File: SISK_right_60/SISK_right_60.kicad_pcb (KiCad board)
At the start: 2 copper layers, 194.5 x 121.8 mm, 76 parts, among them J1 OLED_128x32, J2 Battery Conn, J3 alternative on/off SW (wired), SW1 "6", SW10 "Z", SW11 "U", SW12 "I", SW13 "O", SW14 "P", SW15 "Ü", SW16 "*", SW19 "H", SW2 "7", SW20 "J", SW21 "K", SW22 "L", SW23 "Ö", SW24 "Ä", SW25 "'", SW27 "N", SW28 "M", SW29 ";", SW3 "8", SW30 ":", SW31 "-", SW32 "shift_R", SW35 "SPACE_R", SW36 "Alt", SW37 FN, SW38 "Ctrl", SW39 FN2, SW4 "9", SW5 "0", SW6 "ß", SW7 "`", SW8 "Backspace", SW9 "Enter", U1 Nice_Nano_V2

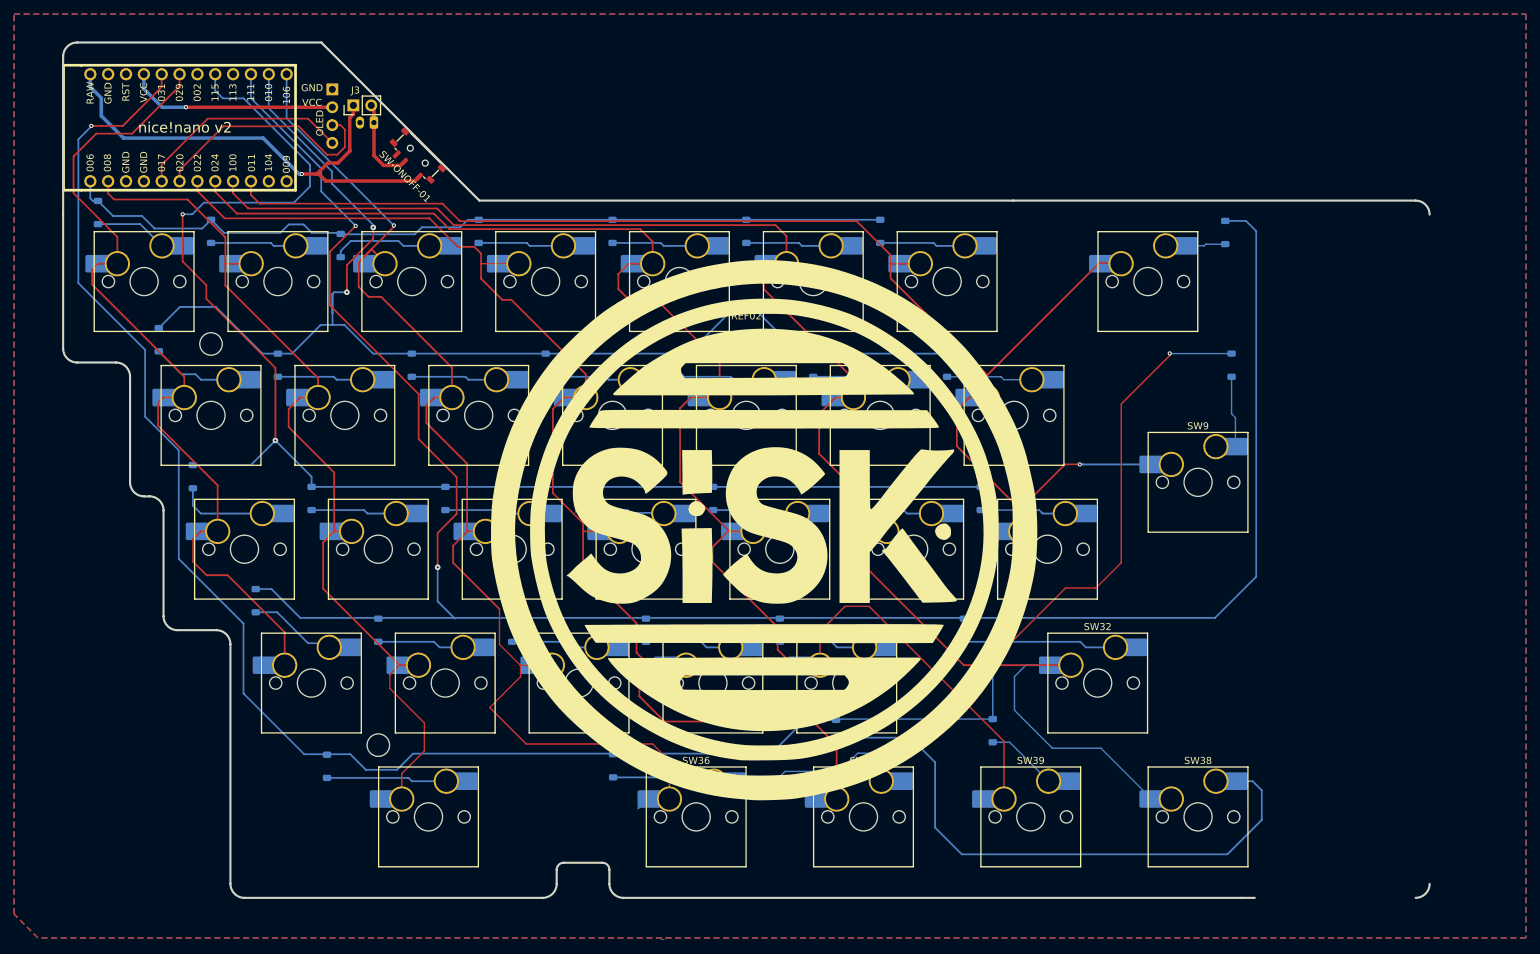
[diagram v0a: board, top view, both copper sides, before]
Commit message: fixed most of issues, updated 60% version
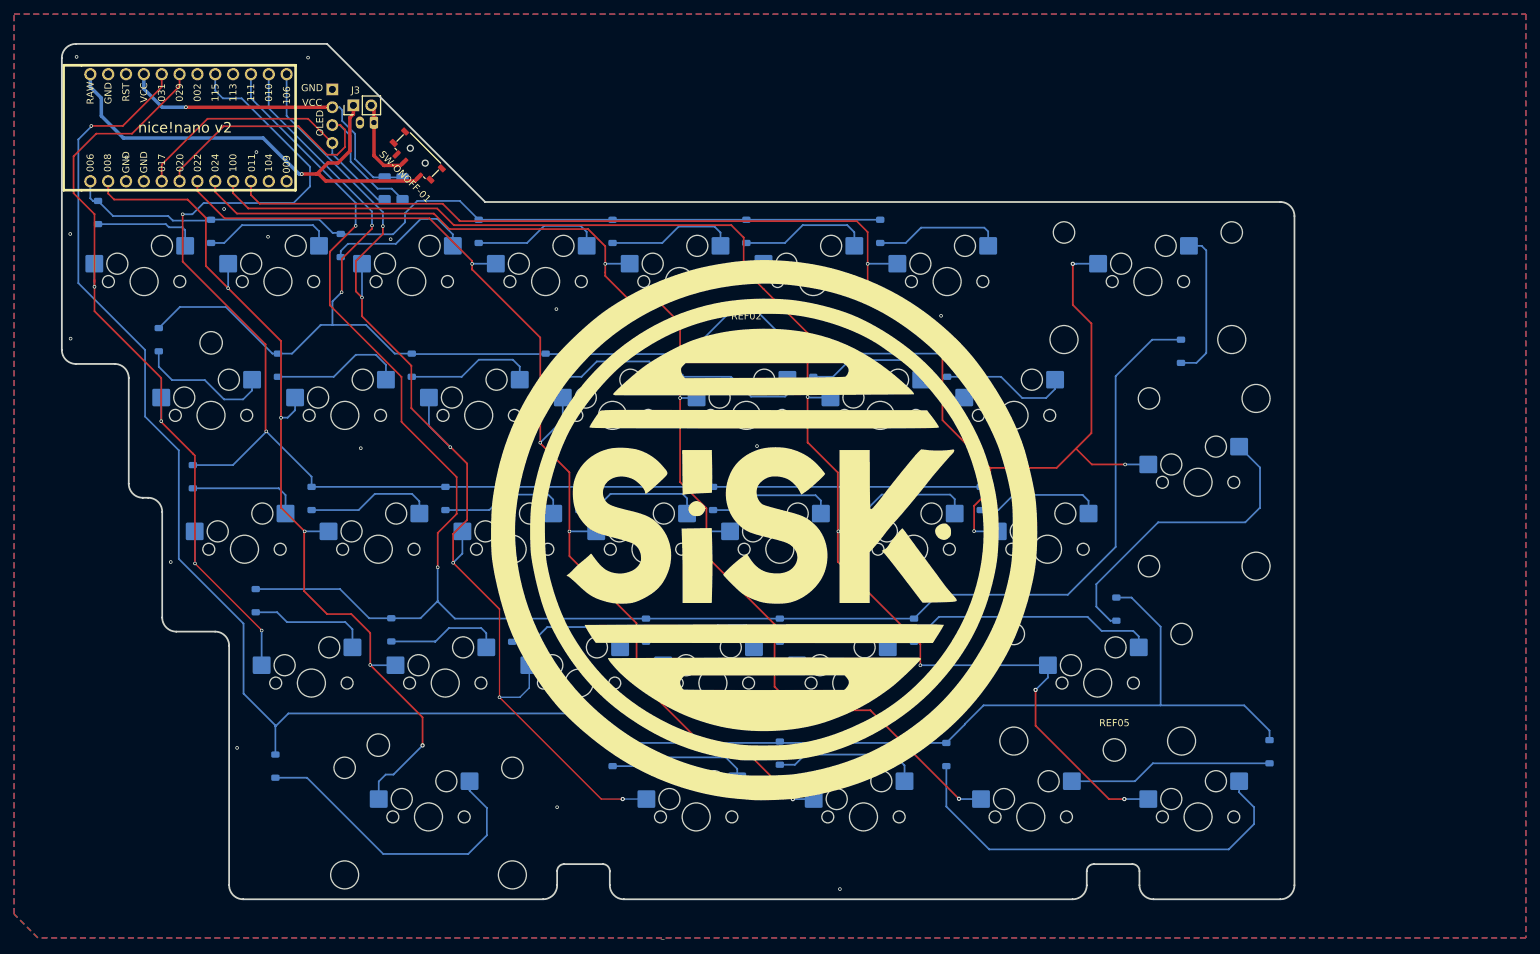
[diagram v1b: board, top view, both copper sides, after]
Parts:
- removed SW39: FN2, ScottoKeebs_Hotswap:Hotswap_MX_Plated_1.25u
- added R1: 5K, Resistor_SMD:R_1206_3216Metric_Pad1.30x1.75mm_HandSolder, B.Cu at (86.7, 51.8)
- added R2: 5K, Resistor_SMD:R_1206_3216Metric_Pad1.30x1.75mm_HandSolder, B.Cu at (89.2, 51.8)
- added REF05: MountingHole_3.2mm_M3_ISO7380, MountingHole:MountingHole_3.2mm_M3_ISO7380, F.Cu at (190.6, 131.7)
- added SW17: SW_push, MX_Hotswap:MX-Hotswap-1.25U, B.Cu at (178.7, 141.2)
- J2: value Battery Conn -> Conn
- J3: value alternative on/off SW (wired) -> SWITCH
- SW-ONOFF-01: value onboard ON/OFF SW -> ~
- SW1: value "6" -> SW_push; footprint ScottoKeebs_Hotswap:Hotswap_MX_Plated_1.00u -> MX_Hotswap:MX-Hotswap-1U; moved to B.Cu
- SW10: value "Z" -> SW_push; footprint ScottoKeebs_Hotswap:Hotswap_MX_Plated_1.00u -> MX_Hotswap:MX-Hotswap-1U; moved to B.Cu
- SW11: value "U" -> SW_push; footprint ScottoKeebs_Hotswap:Hotswap_MX_Plated_1.00u -> MX_Hotswap:MX-Hotswap-1U; moved to B.Cu
- SW12: value "I" -> SW_push; footprint ScottoKeebs_Hotswap:Hotswap_MX_Plated_1.00u -> MX_Hotswap:MX-Hotswap-1U; moved to B.Cu
- SW13: value "O" -> SW_push; footprint ScottoKeebs_Hotswap:Hotswap_MX_Plated_1.00u -> MX_Hotswap:MX-Hotswap-1U; moved to B.Cu
- SW14: value "P" -> SW_push; footprint ScottoKeebs_Hotswap:Hotswap_MX_Plated_1.00u -> MX_Hotswap:MX-Hotswap-1U; moved to B.Cu
- SW15: value "Ü" -> SW_push; footprint ScottoKeebs_Hotswap:Hotswap_MX_Plated_1.00u -> MX_Hotswap:MX-Hotswap-1U; moved to B.Cu
- SW16: value "*" -> SW_push; footprint ScottoKeebs_Hotswap:Hotswap_MX_Plated_1.00u -> MX_Hotswap:MX-Hotswap-1U; moved to B.Cu
- SW19: value "H" -> SW_push; footprint ScottoKeebs_Hotswap:Hotswap_MX_Plated_1.00u -> MX_Hotswap:MX-Hotswap-1U; moved to B.Cu
- SW2: value "7" -> SW_push; footprint ScottoKeebs_Hotswap:Hotswap_MX_Plated_1.00u -> MX_Hotswap:MX-Hotswap-1U; moved to B.Cu
- SW20: value "J" -> SW_push; footprint ScottoKeebs_Hotswap:Hotswap_MX_Plated_1.00u -> MX_Hotswap:MX-Hotswap-1U; moved to B.Cu
- SW21: value "K" -> SW_push; footprint ScottoKeebs_Hotswap:Hotswap_MX_Plated_1.00u -> MX_Hotswap:MX-Hotswap-1U; moved to B.Cu
- SW22: value "L" -> SW_push; footprint ScottoKeebs_Hotswap:Hotswap_MX_Plated_1.00u -> MX_Hotswap:MX-Hotswap-1U; moved to B.Cu
- SW23: value "Ö" -> SW_push; footprint ScottoKeebs_Hotswap:Hotswap_MX_Plated_1.00u -> MX_Hotswap:MX-Hotswap-1U; moved to B.Cu
- SW24: value "Ä" -> SW_push; footprint ScottoKeebs_Hotswap:Hotswap_MX_Plated_1.00u -> MX_Hotswap:MX-Hotswap-1U; moved to B.Cu
- SW25: value "'" -> SW_push; footprint ScottoKeebs_Hotswap:Hotswap_MX_Plated_1.00u -> MX_Hotswap:MX-Hotswap-1U; moved to B.Cu
- SW27: value "N" -> SW_push; footprint ScottoKeebs_Hotswap:Hotswap_MX_Plated_1.00u -> MX_Hotswap:MX-Hotswap-1U; moved to B.Cu
- SW28: value "M" -> SW_push; footprint ScottoKeebs_Hotswap:Hotswap_MX_Plated_1.00u -> MX_Hotswap:MX-Hotswap-1U; moved to B.Cu
- SW29: value ";" -> SW_push; footprint ScottoKeebs_Hotswap:Hotswap_MX_Plated_1.00u -> MX_Hotswap:MX-Hotswap-1U; moved to B.Cu
- SW3: value "8" -> SW_push; footprint ScottoKeebs_Hotswap:Hotswap_MX_Plated_1.00u -> MX_Hotswap:MX-Hotswap-1U; moved to B.Cu
- SW30: value ":" -> SW_push; footprint ScottoKeebs_Hotswap:Hotswap_MX_Plated_1.00u -> MX_Hotswap:MX-Hotswap-1U; moved to B.Cu
- SW31: value "-" -> SW_push; footprint ScottoKeebs_Hotswap:Hotswap_MX_Plated_1.00u -> MX_Hotswap:MX-Hotswap-1U; moved to B.Cu
- SW32: value "shift_R" -> SW_push; footprint ScottoKeebs_Hotswap:Hotswap_MX_Plated_2.75u -> MX_Hotswap:MX-Hotswap-2.75U; moved to B.Cu
- SW35: value "SPACE_R" -> SW_push; footprint ScottoKeebs_Hotswap:Hotswap_MX_Plated_2.75u -> MX_Hotswap:MX-Hotswap-2.75U; moved to B.Cu
- SW36: value "Alt" -> SW_push; footprint ScottoKeebs_Hotswap:Hotswap_MX_Plated_1.25u -> MX_Hotswap:MX-Hotswap-1.25U; moved to B.Cu
- SW37: value FN -> SW_push; footprint ScottoKeebs_Hotswap:Hotswap_MX_Plated_1.25u -> MX_Hotswap:MX-Hotswap-1.25U; moved to B.Cu
- SW38: value "Ctrl" -> SW_push; footprint ScottoKeebs_Hotswap:Hotswap_MX_Plated_1.25u -> MX_Hotswap:MX-Hotswap-1.25U; moved to B.Cu
- SW4: value "9" -> SW_push; footprint ScottoKeebs_Hotswap:Hotswap_MX_Plated_1.00u -> MX_Hotswap:MX-Hotswap-1U; moved to B.Cu
- SW5: value "0" -> SW_push; footprint ScottoKeebs_Hotswap:Hotswap_MX_Plated_1.00u -> MX_Hotswap:MX-Hotswap-1U; moved to B.Cu
- SW6: value "ß" -> SW_push; footprint ScottoKeebs_Hotswap:Hotswap_MX_Plated_1.00u -> MX_Hotswap:MX-Hotswap-1U; moved to B.Cu
- SW7: value "`" -> SW_push; footprint ScottoKeebs_Hotswap:Hotswap_MX_Plated_1.00u -> MX_Hotswap:MX-Hotswap-1U; moved to B.Cu
- SW8: value "Backspace" -> SW_push; footprint ScottoKeebs_Hotswap:Hotswap_MX_Plated_2.00u -> MX_Hotswap:MX-Hotswap-2U; moved to B.Cu
- SW9: value "Enter" -> SW_push; footprint ScottoKeebs_Hotswap:Hotswap_MX_Plated_ISOEnter -> MX_Hotswap:MX-Hotswap-ISO; moved to B.Cu
- moved D3 39.5 mm to (212.6, 131.9)
- moved D2 38.4 mm to (190.8, 111.6)
- moved D1 18.0 mm to (200.0, 74.9)
- moved D25 16.0 mm to (166.6, 132.3)
- moved D8 7.35 mm to (71.1, 134.0)
- moved D19 7.09 mm to (162.0, 114.6)
- moved D30 2.02 mm to (142.9, 132.1)
- moved D39 1.85 mm to (87.6, 114.6)
- moved D35 1.60 mm to (119.1, 132.3)
- moved REF01 0.16 mm to (62.0, 73.7)
- turned SW1 to 180 degrees
- turned SW10 to 180 degrees
- turned SW11 to 180 degrees
- turned SW12 to 180 degrees
- turned SW13 to 180 degrees
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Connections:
- net +3.3V renamed +BATT
- net Net-(J1-SCL) renamed /SCL
- net Net-(J1-SDA) renamed /SDA
- net Net-(J3-Pin_1) renamed +VDC
- net VCC renamed +3,3V
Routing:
- net /ROW3: track 295.5 -> 257.5 mm
- net Net-(D2-A): track 10.2 -> 44.6 mm
- net /COL4: track 212.3 -> 183.9 mm, vias 0 -> 5
- net Net-(D8-A): track 17.8 -> 44.4 mm
- net Net-(D25-A): track 83.8 -> 60.6 mm
- net /COL5: track 226.6 -> 206.0 mm, vias 0 -> 6
- net Net-(D3-A): track 10.3 -> 29.2 mm
- net +3,3V: track 30.1 -> 47.4 mm
- net /SCL: track 34.4 -> 50.9 mm
- net /COL3: track 180.4 -> 165.0 mm, vias 0 -> 5
- net Net-(D1-A): track 6.92 -> 21.5 mm
- net Net-(D19-A): track 21.9 -> 36.2 mm
- net /COL2: track 171.3 -> 159.3 mm, vias 1 -> 6
- net /SDA: track 30.8 -> 42.5 mm
- net /ROW4: track 294.6 -> 284.3 mm, vias 3 -> 1
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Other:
- board size 194.5 x 121.8 mm -> 175.4 x 121.8 mm
